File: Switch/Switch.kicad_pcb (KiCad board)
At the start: 2 copper layers, 22.1 x 128.4 mm, 19 parts, among them SW1 SW_SPDT, SW2 SW_SPDT

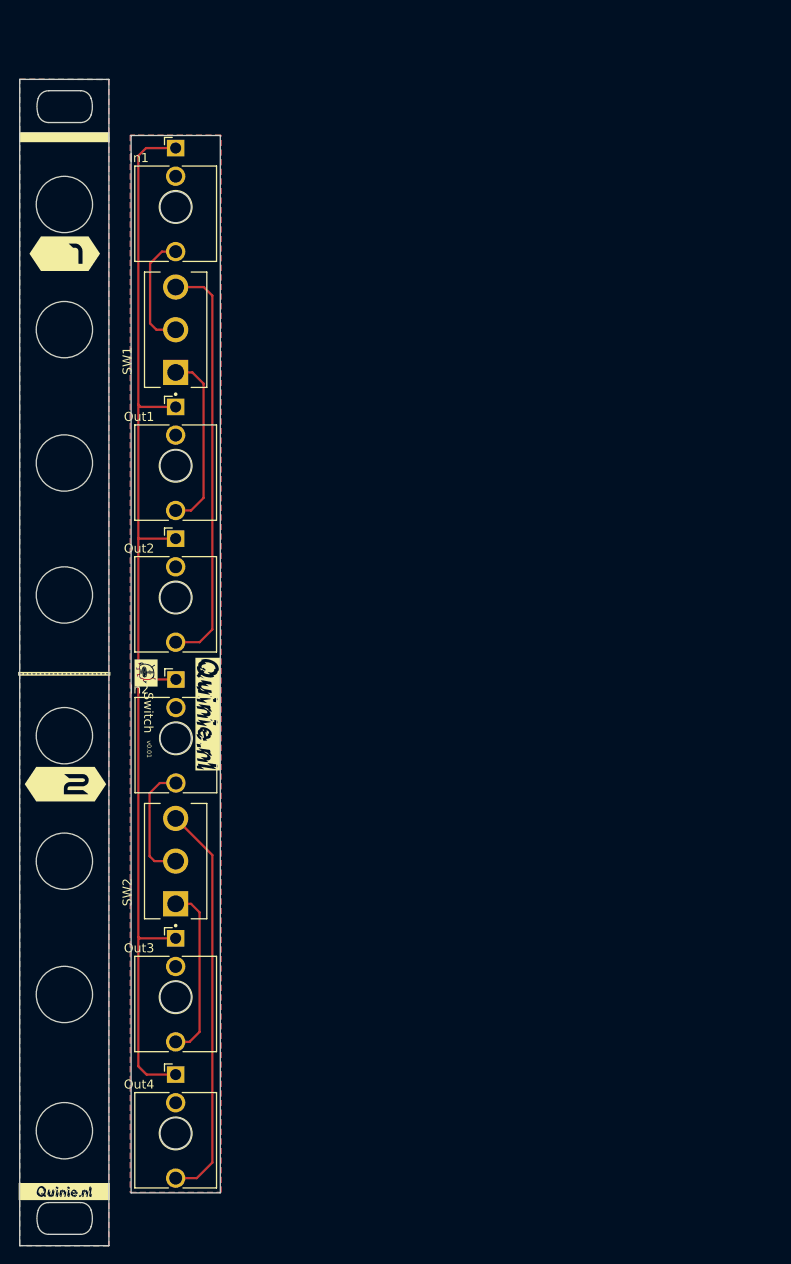
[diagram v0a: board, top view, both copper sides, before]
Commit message: Updates
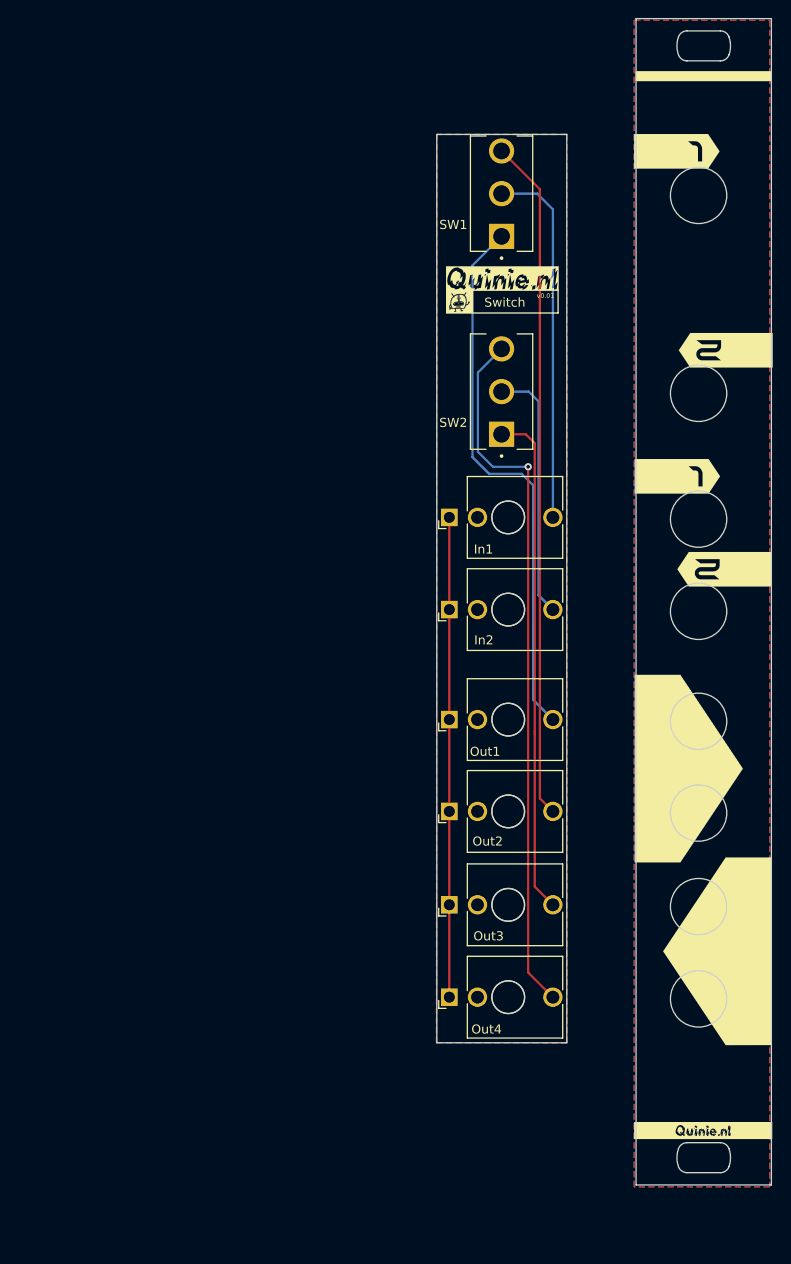
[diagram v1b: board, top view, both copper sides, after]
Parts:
- removed the kibuzzard-63663374 at (38.0, 84.3)
- removed the kibuzzard-63663374 at (44.7, 84.1)
- removed the kibuzzard-63663374 at (32.4, 79.2)
- removed the kibuzzard-63729A5C at (44.8, 88.8)
- removed the kibuzzard-63729A5C at (25.4, 83.4)
- removed the kibuzzard-63729A5C at (38.0, 88.6)
- removed kibuzzard-6564E20D: G***, kibuzzard-6564E20D
- removed kibuzzard-6564E26E: G***, kibuzzard-6564E26E
- removed kibuzzard-6564E2EE: G***, kibuzzard-6564E2EE
- removed kibuzzard-65663047: G***, kibuzzard-65663047
- removed kibuzzard-65663061: G***, kibuzzard-65663061
- added REF**: KiCad-Logo2_5mm_SilkScreen, Symbol:KiCad-Logo2_5mm_SilkScreen, B.Cu at (95.3, 42.1)
- added REF**: ESD-Logo_6.6x6mm_SilkScreen, Symbol:ESD-Logo_6.6x6mm_SilkScreen, B.Cu at (102.7, 49.6)
- added REF**: WEEE-Logo_4.2x6mm_SilkScreen, Symbol:WEEE-Logo_4.2x6mm_SilkScreen, B.Cu at (102.7, 36.9)
- added REF**: OSHW-Logo2_7.3x6mm_SilkScreen, Symbol:OSHW-Logo2_7.3x6mm_SilkScreen, B.Cu at (103.0, 42.5)
- added kibuzzard-63663374: G***, kibuzzard-63663374, F.Cu at (72.5, 43.5)
- added kibuzzard-63663374: G***, kibuzzard-63663374, B.Cu at (81.9, 43.5)
- added kibuzzard-63729A5C: G***, kibuzzard-63729A5C, F.Cu at (77.2, 40.9)
- added kibuzzard-63729A5C: G***, kibuzzard-63729A5C, B.Cu at (77.2, 40.9)
- added kibuzzard-63920CDF: G***, kibuzzard-63920CDF, F.Cu at (128.0, 114.9)
- added kibuzzard-63920CDF: G***, kibuzzard-63920CDF, F.Cu at (70.6, 94.8)
- added kibuzzard-63948EC7: G***, kibuzzard-63948EC7, F.Cu at (101.8, 48.8)
- added kibuzzard-63948EC7: G***, kibuzzard-63948EC7, F.Cu at (101.7, 72.9)
- added kibuzzard-63948EE9: G***, kibuzzard-63948EE9, F.Cu at (96.5, 62.6)
- added kibuzzard-63948EE9: G***, kibuzzard-63948EE9, F.Cu at (96.4, 26.9)
- added kibuzzard-656B60C2: G***, kibuzzard-656B60C2, F.Cu at (99.3, 134.7)
- added kibuzzard-656B617B: G***, kibuzzard-656B617B, B.Cu at (99.3, 24.4)
- added kibuzzard-656C56A9: G***, kibuzzard-656C56A9, F.Cu at (99.4, 132.4)
- moved SW2 62.9 mm to (77.1, 53.3)
- moved In1 50.6 mm to (71.4, 67.2), turned to 90 degrees
- moved Out1 45.7 mm to (71.4, 89.4), turned to 90 degrees
- moved Out2 42.5 mm to (71.4, 99.5), turned to 90 degrees
- moved SW1 38.9 mm to (77.1, 31.5)
- moved Out4 31.3 mm to (71.4, 120.0), turned to 90 degrees
- moved In2 31.1 mm to (71.4, 77.3), turned to 90 degrees
- moved Out3 30.4 mm to (71.4, 109.8), turned to 90 degrees
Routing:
- net GND: track 125.9 -> 52.8 mm
- net Net-(SW1-A): track 19.8 -> 60.3 mm
- net Net-(SW2-A): track 19.3 -> 56.0 mm
- net Net-(SW2-C): track 44.3 -> 78.1 mm, vias 0 -> 1
- net Net-(SW1-C): track 45.8 -> 75.1 mm
- net Net-(SW1-B): track 13.1 -> 40.3 mm
- net Net-(SW2-B): track 13.4 -> 28.1 mm
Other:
- board size 22.1 x 128.4 mm -> 36.8 x 128.4 mm
- board text added: "JLCJLCJLCJLC"
